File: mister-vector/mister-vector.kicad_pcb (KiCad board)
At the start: 4 copper layers, 68.6 x 106.6 mm, 120 parts, among them IC5 TL084, IC7 TL084, J2 AUDIO_JACK_3.5MM_KIT, U1 VASD1-SIP, U2 SN74LVC821ADGVR, U3 SN74LVC821ADGVR, U4 SN74LVC821ADGVR

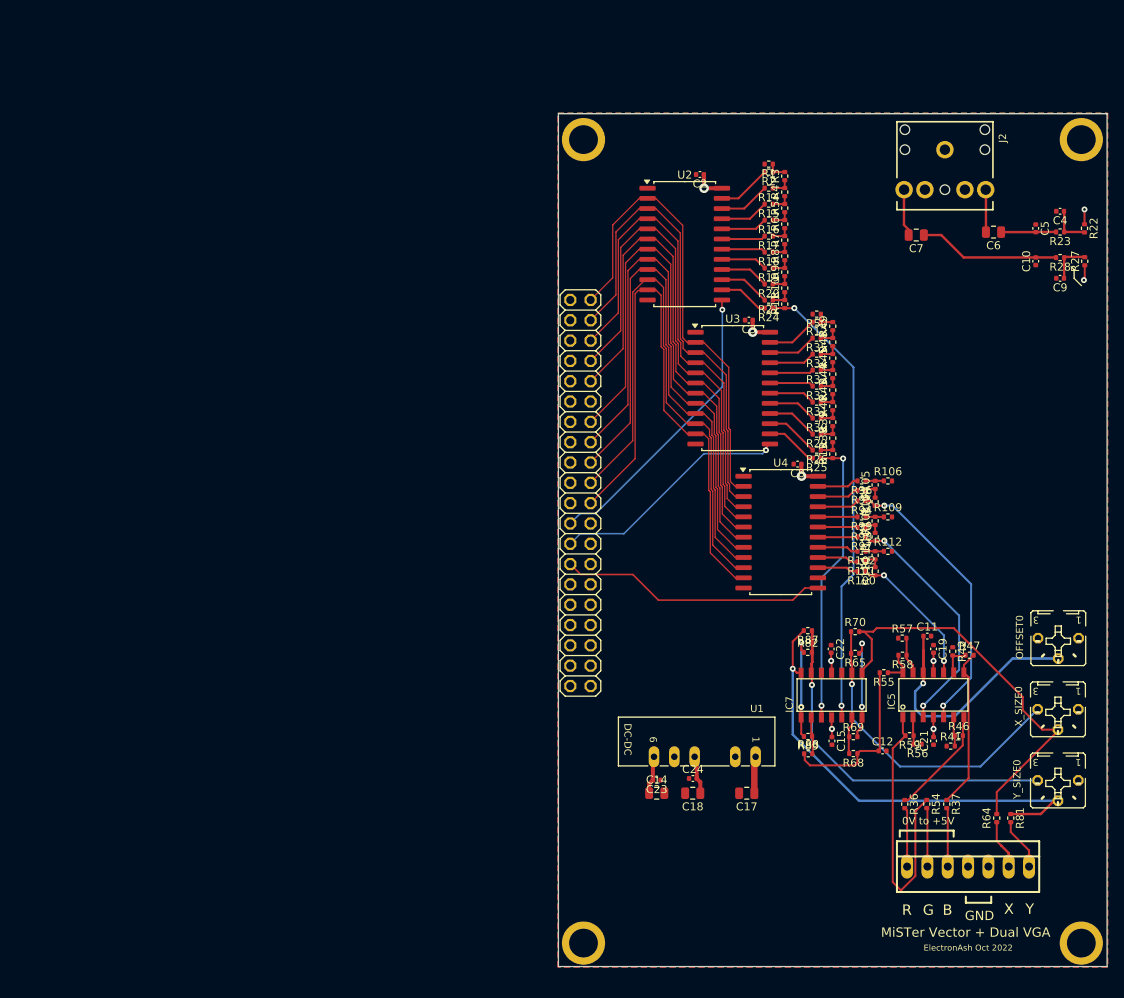
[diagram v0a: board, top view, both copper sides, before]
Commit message: update pcb screenshot
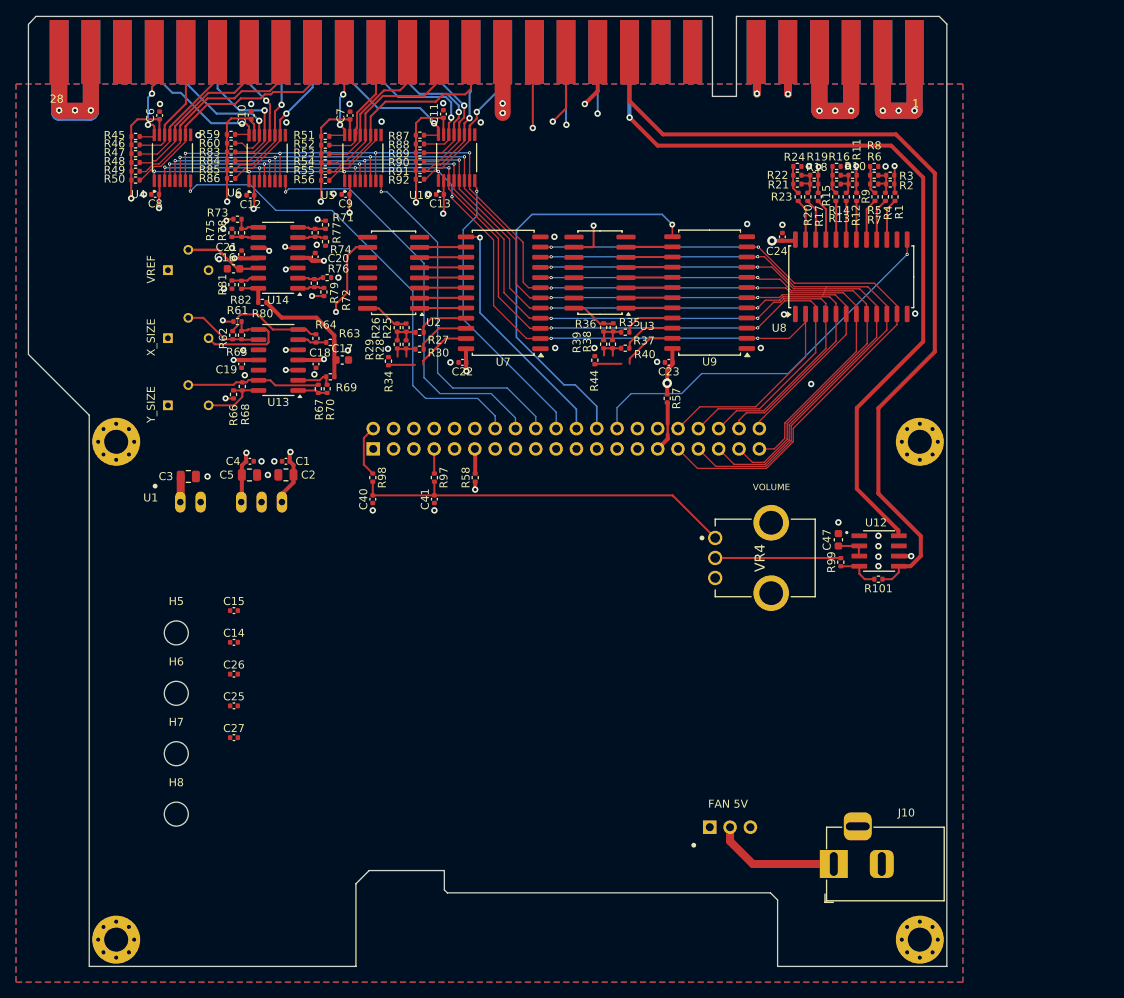
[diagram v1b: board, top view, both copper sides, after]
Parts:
- removed GPIO1: PINHD-2X20, 2X20
- removed IC5, IC7: TL084, SOIC-14
- removed J2: AUDIO_JACK_3.5MM_KIT, AUDIO-JACK-KIT
- removed OFFSET0, X_SIZE0, Y_SIZE0: 20K, B25P
- removed R100, R102, R106, R109, R112, R31, R32, R33, R94, R95, R96: 2k, Resistor_SMD:R_0402_1005Metric
- removed R104, R105, R107, R108, R110, R111, R43: 1k, Resistor_SMD:R_0402_1005Metric
- removed R41, R42: 10K, Resistor_SMD:R_0402_1005Metric
- removed U$1, U$2, U$3, U$4: PLATED_HOLE3.6MM, PLATED_HOLE_3.6MM
- removed VEC_OUT1: 22-23-2071, 22-23-2071
- added C1: 100nF, Capacitor_SMD:C_0402_1005Metric, F.Cu at (80.1, 95.1)
- added C13: 100nF, Capacitor_SMD:C_0402_1005Metric, F.Cu at (99.4, 61.8)
- added C16: 1uF, Capacitor_SMD:C_0603_1608Metric, F.Cu at (73.6, 71.1)
- added C20: 100nF, Capacitor_SMD:C_0402_1005Metric, F.Cu at (83.8, 69.6)
- added C25: 0.1pF, Capacitor_SMD:C_0402_1005Metric, F.Cu at (73.7, 125.7)
- added C26: 0.1pF, Capacitor_SMD:C_0402_1005Metric, F.Cu at (73.7, 121.8)
- added C27: 0.1pF, Capacitor_SMD:C_0402_1005Metric, F.Cu at (73.7, 129.7)
- added C40: 20nF, Capacitor_SMD:C_0402_1005Metric, F.Cu at (91.0, 99.9)
- added C41: 20nF, Capacitor_SMD:C_0402_1005Metric, F.Cu at (98.7, 99.9)
- added C47: 1uF, Capacitor_SMD:C_0603_1608Metric, F.Cu at (149.2, 105.0)
- added G***: LOGO, LOGO, F.Cu at (53.6, 56.7)
- added H1: MountingHole_Pad, MountingHole:MountingHole_3mm_Pad_Via, F.Cu at (159.4, 154.9)
- added H2: MountingHole_Pad, MountingHole:MountingHole_3mm_Pad_Via, F.Cu at (58.9, 92.7)
- added H3: MountingHole_Pad, MountingHole:MountingHole_3mm_Pad_Via, F.Cu at (159.4, 92.7)
- added H4: MountingHole_Pad, MountingHole:MountingHole_3mm_Pad_Via, F.Cu at (58.9, 154.9)
- added H5: FAN1, MountingHole:MountingHole_3mm, F.Cu at (66.4, 116.6)
- added H6: FAN2, MountingHole:MountingHole_3mm, F.Cu at (66.4, 124.2)
- added H7: FAN3, MountingHole:MountingHole_3mm, F.Cu at (66.4, 131.7)
- added H8: FAN4, MountingHole:MountingHole_3mm, F.Cu at (66.4, 139.2)
- added J10: DC-005-2.5A-2.0 C319099, Connector_BarrelJack:BarrelJack_Horizontal, F.Cu at (148.6, 145.5)
- added J100: FAN, Connector_PinHeader_2.54mm:PinHeader_1x03_P2.54mm_Vertical, F.Cu at (133.1, 140.9)
- added J7: PINHD-2X20, Connector_PinSocket_2.54mm:PinSocket_2x20_P2.54mm_Vertical, B.Cu at (91.1, 93.6)
- added J8: Jamma_con, Jamma:JAMMA-56, F.Cu at (158.9, 43.9)
- added R51: 100k, Resistor_SMD:R_0402_1005Metric, F.Cu at (85.1, 54.5)
- added R52: 100k, Resistor_SMD:R_0402_1005Metric, F.Cu at (85.1, 55.6)
- added R53: 100k, Resistor_SMD:R_0402_1005Metric, F.Cu at (85.1, 56.7)
- added R60: 100k, Resistor_SMD:R_0402_1005Metric, F.Cu at (73.3, 55.4)
- added R61: 75R, Resistor_SMD:R_0402_1005Metric, F.Cu at (74.1, 77.7)
- added R62: 75R, Resistor_SMD:R_0402_1005Metric, F.Cu at (73.5, 79.4)
- added R63: 10K, Resistor_SMD:R_0402_1005Metric, F.Cu at (85.7, 80.3)
- added R66: 75R, Resistor_SMD:R_0402_1005Metric, F.Cu at (73.6, 86.8)
- added R67: 75R, Resistor_SMD:R_0402_1005Metric, F.Cu at (84.2, 86.1)
- added R71: 75R, Resistor_SMD:R_0402_1005Metric, F.Cu at (85.1, 65.6)
- added R72: 75R, Resistor_SMD:R_0402_1005Metric, F.Cu at (84.9, 74.0)
- added R73: 75R, Resistor_SMD:R_0402_1005Metric, F.Cu at (74.1, 64.9)
- added R74: 10K, Resistor_SMD:R_0402_1005Metric, F.Cu at (85.1, 67.7)
- added R75: 10K, Resistor_SMD:R_0402_1005Metric, F.Cu at (73.4, 66.6)
- added R76: 10K, Resistor_SMD:R_0402_1005Metric, F.Cu at (85.3, 72.2)
- added R77: 4K7, Resistor_SMD:R_0402_1005Metric, F.Cu at (83.8, 66.6)
- added R78: 4K7, Resistor_SMD:R_0402_1005Metric, F.Cu at (74.6, 66.6)
- added R79: 4K7, Resistor_SMD:R_0402_1005Metric, F.Cu at (83.7, 72.9)
- added R80: 75R, Resistor_SMD:R_0402_1005Metric, F.Cu at (77.2, 75.3)
- added R83: 100k, Resistor_SMD:R_0402_1005Metric, F.Cu at (73.3, 56.5)
- added R84: 100k, Resistor_SMD:R_0402_1005Metric, F.Cu at (73.3, 57.6)
- added R85: 100k, Resistor_SMD:R_0402_1005Metric, F.Cu at (73.3, 58.7)
- added R86: 100k, Resistor_SMD:R_0402_1005Metric, F.Cu at (73.3, 59.8)
- added R90: 100k, Resistor_SMD:R_0402_1005Metric, F.Cu at (96.9, 57.7)
- added R91: 100k, Resistor_SMD:R_0402_1005Metric, F.Cu at (96.9, 58.8)
- added R92: 100k, Resistor_SMD:R_0402_1005Metric, F.Cu at (96.9, 59.9)
- added U10: TXB0106PWR, TXB0106PWR:SOP65P640X120-16N, F.Cu at (101.5, 57.2)
- added U12: LM4871MX_NOPB, LM4871MX_NOPB:SOIC127P599X175-8N, F.Cu at (154.3, 106.4)
- added U13: TL084HIDR, Package_SO:SOIC-14_3.9x8.7mm_P1.27mm, F.Cu at (79.2, 82.5)
- added U14: TL084HIDR, Package_SO:SOIC-14_3.9x8.7mm_P1.27mm, F.Cu at (79.2, 69.7)
- added U5: TXB0106PWR, TXB0106PWR:SOP65P640X120-16N, F.Cu at (89.8, 57.2)
- added U6: TXB0106PWR, TXB0106PWR:SOP65P640X120-16N, F.Cu at (77.8, 57.3)
- added U7: SN74LVC821ADGVR, Package_SO:SOIC-24W_7.5x15.4mm_P1.27mm, F.Cu at (107.3, 74.1)
- added U8: SN74LVC821ADGVR, Package_SO:SOIC-24W_7.5x15.4mm_P1.27mm, F.Cu at (150.8, 72.1)
- added U9: SN74LVC821ADGVR, Package_SO:SOIC-24W_7.5x15.4mm_P1.27mm, F.Cu at (133.1, 74.1)
- added VR1: VREF, 3362P_1_203LF:TRIM_3362P-1-203LF, F.Cu at (67.9, 71.3)
- added VR2: X_SIZE, 3362P_1_203LF:TRIM_3362P-1-203LF, F.Cu at (67.9, 79.8)
- added VR3: Y_SIZE, 3362P_1_203LF:TRIM_3362P-1-203LF, F.Cu at (67.9, 88.2)
- added VR4: 50k, PTV09A-4020U-A503:PTV09A4020FB103, F.Cu at (139.4, 107.2)
- C10, C4, C9: value 10nF -> 100nF
- C11, C12: value 1.0uF -> 100nF
- C14: value 4.7uF -> 0.1pF; footprint Capacitor_SMD:C_0805_2012Metric -> Capacitor_SMD:C_0402_1005Metric
- C15: value 100nF -> 0.1pF
- C17: value 4.7uF -> 1uF; footprint Capacitor_SMD:C_0805_2012Metric -> Capacitor_SMD:C_0603_1608Metric
- C18: value 4.7uF -> 100nF; footprint Capacitor_SMD:C_0805_2012Metric -> Capacitor_SMD:C_0402_1005Metric
- C2, C3: value 100nF -> 4.7uF; footprint Capacitor_SMD:C_0402_1005Metric -> Capacitor_SMD:C_0805_2012Metric
- C5: value 10nF -> 4.7uF; footprint Capacitor_SMD:C_0402_1005Metric -> Capacitor_SMD:C_0805_2012Metric
- C6, C7: value 4.7uF BP -> 100nF; footprint Capacitor_SMD:C_0805_2012Metric -> Capacitor_SMD:C_0402_1005Metric
- R1, R12, R14, R15, R16, R17, R18, R19, R2, R20, R21, R24, R25, R26, R29, R30, R34, R35: value 2k -> 100k 0.1%
- R10, R11, R13, R3, R38, R39, R4, R40, R44, R5, R6, R7, R8, R9: value 1k -> 100k 0.1%
- R101, R99: value 2k -> 20k
- R22, R23, R27, R28: value 510R -> 100k 0.1%
- R36, R37: value 75R -> 100k 0.1%
- R45, R48, R49: value 1k -> 100k
- R46, R47, R59: value 4K7 -> 100k
- R50: value 2k -> 100k
- R54, R55: value 75R -> 100k
- R56, R87, R88, R89: value 10K -> 100k
- R57: value 10K -> 0
- R58: value 4K7 -> 0
- R64, R65, R81: value 75R -> 10K
- R82: value 75R -> 4K7
- R97, R98: value 2k -> 475R
- U1: value VASD1-SIP -> RD-0512D
- U2, U3: value SN74LVC821ADGVR -> 4816P-R2R-503LF; footprint Package_SO:SOIC-24W_7.5x15.4mm_P1.27mm -> Package_SO:SOIC-16W_5.3x10.2mm_P1.27mm
- U4: value SN74LVC821ADGVR -> TXB0106PWR; footprint Package_SO:SOIC-24W_7.5x15.4mm_P1.27mm -> TXB0106PWR:SOP65P640X120-16N
- moved R46 126.7 mm to (61.4, 55.6), turned to 180 degrees
- moved R47 121.6 mm to (61.4, 56.7), turned to 180 degrees
- moved R81 118.0 mm to (73.4, 73.1), turned to 90 degrees
- moved R59 113.3 mm to (73.3, 54.3)
- moved R54 109.9 mm to (85.1, 57.8), turned to 180 degrees
- moved C4 106.0 mm to (75.6, 95.1)
- moved C21 105.7 mm to (74.6, 69.3), turned to -90 degrees
- moved C6 105.3 mm to (64.4, 51.9), turned to 90 degrees
- moved C12 105.2 mm to (75.7, 61.9), turned to 180 degrees
- moved R64 104.1 mm to (83.9, 79.8), turned to 90 degrees
- moved C5 103.0 mm to (75.6, 96.9), turned to 0 degrees
- moved R56 102.2 mm to (85.1, 60.0)
- moved C10 99.8 mm to (75.8, 51.9)
- moved R55 93.8 mm to (85.1, 58.9)
- moved C19 93.5 mm to (74.6, 83.0), turned to 90 degrees
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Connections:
- C10 pad 1: GND -> +5V
- C10 pad 2: Net-(C10-Pad2) -> GND
- C11 pad 1: Net-(IC5D-+IN) -> +5V
- C12 pad 1: /+VREF -> +3.3V
- C14 pad 1: +12V -> GND
- C14 pad 2: GND -> /Vector Amplifiers/DAC_B
- C15 pad 1: +12V -> GND
- C15 pad 2: GND -> /Vector Amplifiers/DAC_G
- C17 pad 1: +5V -> /Vector Amplifiers/+VREF
- C18 pad 1: -12V -> GND
- C18 pad 2: GND -> +12V
- C2 pad 1: +3.3V -> +12V
- C21 pad 2: +12V -> -12V
- C22 pad 1: GND -> +3.3V
- C22 pad 2: -12V -> GND
- C23 pad 1: GND -> +3.3V
- C23 pad 2: +12V -> GND
- C24 pad 1: GND -> +3.3V
- C24 pad 2: -12V -> GND
- C3 pad 1: +3.3V -> +5V
- C4 pad 1: Net-(C4-Pad1) -> GND
- C4 pad 2: GND -> -12V
- C5 pad 1: GND -> -12V
- C5 pad 2: Net-(C5-Pad2) -> GND
- C6 pad 1: Net-(C5-Pad2) -> +5V
- C6 pad 2: Net-(C6-Pad2) -> GND
- C7 pad 1: Net-(C10-Pad2) -> +5V
- C7 pad 2: Net-(C7-Pad2) -> GND
- C9 pad 1: Net-(C9-Pad1) -> +3.3V
- R1 pad 1: Net-(R1-Pad1) -> /Vector Amplifiers/DAC_B
- R1 pad 2: GND -> /Vector DACs/R2R_DAC_B/D2
- R10 pad 1: Net-(R10-Pad1) -> /Vector Amplifiers/DAC_G
- R101 pad 1: Net-(R101-Pad1) -> /JAMMA_SPEAKER+
- R101 pad 2: /R2R_DAC_B/D1 -> Net-(U12--IN)
- R11 pad 1: /DAC_X -> /Vector Amplifiers/DAC_G
- R11 pad 2: Net-(R10-Pad1) -> Net-(R10-Pad2)
- R12 pad 1: Net-(R12-Pad1) -> Net-(R10-Pad2)
- R12 pad 2: /R2R_DAC_Y/D0 -> /Vector DACs/R2R_DAC_G/D1
- R13 pad 1: /DAC_Y -> Net-(R10-Pad2)
- R14 pad 1: Net-(R14-Pad1) -> Net-(R10-Pad2)
- R14 pad 2: /R2R_DAC_X/D1 -> Net-(R13-Pad2)
- R15 pad 1: Net-(R15-Pad1) -> Net-(R13-Pad2)
- R15 pad 2: /R2R_DAC_X/D2 -> /Vector DACs/R2R_DAC_G/D0
- R16 pad 1: Net-(R16-Pad1) -> Net-(R13-Pad2)
- R16 pad 2: /R2R_DAC_X/D3 -> GND
- R17 pad 1: Net-(R17-Pad1) -> /Vector Amplifiers/DAC_R
- R17 pad 2: /R2R_DAC_X/D4 -> /Vector DACs/R2R_DAC_R/D2
- R18 pad 1: Net-(R18-Pad1) -> /Vector Amplifiers/DAC_R
- R18 pad 2: /R2R_DAC_X/D5 -> Net-(R18-Pad2)
- R19 pad 1: Net-(R19-Pad1) -> /Vector Amplifiers/DAC_R
- R19 pad 2: /R2R_DAC_X/D6 -> Net-(R18-Pad2)
- R2 pad 1: Net-(R1-Pad1) -> /Vector Amplifiers/DAC_B
- R2 pad 2: /R2R_DAC_X/D0 -> Net-(R2-Pad2)
- R20 pad 1: Net-(R10-Pad2) -> Net-(R18-Pad2)
- R20 pad 2: /R2R_DAC_X/D7 -> /Vector DACs/R2R_DAC_R/D1
- R21 pad 1: Net-(R10-Pad1) -> Net-(R18-Pad2)
- R21 pad 2: /R2R_DAC_X/D8 -> Net-(R21-Pad2)
- R22 pad 1: /AUDIO_R -> Net-(R18-Pad2)
- R22 pad 2: Net-(C4-Pad1) -> Net-(R21-Pad2)
- R23 pad 1: Net-(C4-Pad1) -> Net-(R21-Pad2)
- R23 pad 2: Net-(C5-Pad2) -> /Vector DACs/R2R_DAC_R/D0
- R24 pad 1: /DAC_X -> Net-(R21-Pad2)
- R24 pad 2: /R2R_DAC_X/D9 -> GND
- R25 pad 1: /DAC_Y -> Net-(R25-Pad1)
- R25 pad 2: /R2R_DAC_Y/D9 -> Net-(R25-Pad2)
- R26 pad 1: Net-(R13-Pad2) -> Net-(R25-Pad1)
- R26 pad 2: /R2R_DAC_Y/D8 -> Net-(R25-Pad2)
- R27 pad 1: /AUDIO_L -> Net-(R25-Pad2)
- R27 pad 2: Net-(C9-Pad1) -> /Vector DACs/R2R_DAC_X/D1
- R28 pad 1: Net-(C9-Pad1) -> Net-(R25-Pad2)
- R28 pad 2: Net-(C10-Pad2) -> Net-(R28-Pad2)
- R29 pad 1: Net-(R29-Pad1) -> Net-(R25-Pad2)
- R29 pad 2: /R2R_DAC_Y/D7 -> Net-(R28-Pad2)
- R3 pad 1: Net-(R14-Pad1) -> /Vector Amplifiers/DAC_B
- R3 pad 2: Net-(R1-Pad1) -> Net-(R2-Pad2)
- R30 pad 1: Net-(R30-Pad1) -> Net-(R28-Pad2)
- R30 pad 2: /R2R_DAC_Y/D6 -> /Vector DACs/R2R_DAC_X/D0
- R34 pad 1: Net-(R34-Pad1) -> Net-(R28-Pad2)
- R34 pad 2: /R2R_DAC_Y/D2 -> GND
- R35 pad 2: /R2R_DAC_Y/D1 -> Net-(R35-Pad2)
- R36 pad 1: Net-(IC5B-OUT) -> Net-(R35-Pad1)
- R36 pad 2: /R -> Net-(R35-Pad2)
- R37 pad 1: Net-(IC5C-OUT) -> Net-(R35-Pad2)
- R37 pad 2: /B -> /Vector DACs/R2R_DAC_Y/D1
- R38 pad 1: Net-(R13-Pad2) -> Net-(R35-Pad2)
- R38 pad 2: Net-(R29-Pad1) -> Net-(R38-Pad2)
- R39 pad 1: Net-(R29-Pad1) -> Net-(R35-Pad2)
- R39 pad 2: Net-(R30-Pad1) -> Net-(R38-Pad2)
- R4 pad 1: Net-(R15-Pad1) -> Net-(R2-Pad2)
- R4 pad 2: Net-(R14-Pad1) -> /Vector DACs/R2R_DAC_B/D1
- R40 pad 1: Net-(R30-Pad1) -> Net-(R38-Pad2)
- R40 pad 2: Net-(R31-Pad1) -> /Vector DACs/R2R_DAC_Y/D0
- R44 pad 1: Net-(R32-Pad1) -> Net-(R38-Pad2)
- R44 pad 2: Net-(R33-Pad1) -> GND
- R45 pad 1: Net-(R33-Pad1) -> /JAMMA_P1_BUTTON4
- R45 pad 2: Net-(R34-Pad1) -> +5V
- R46 pad 1: Net-(IC5B--IN) -> /JAMMA_P1_BUTTON3
- R46 pad 2: Net-(IC5B-OUT) -> +5V
- R47 pad 1: Net-(IC5C--IN) -> /JAMMA_P1_BUTTON2
- R47 pad 2: Net-(IC5C-OUT) -> +5V
- R48 pad 1: Net-(R34-Pad1) -> /JAMMA_P1_BUTTON1
- R48 pad 2: Net-(R35-Pad1) -> +5V
- R49 pad 1: Net-(R35-Pad1) -> /JAMMA_P1_R
- R49 pad 2: Net-(R12-Pad1) -> +5V
- R5 pad 1: Net-(R16-Pad1) -> Net-(R2-Pad2)
- R5 pad 2: Net-(R15-Pad1) -> Net-(R5-Pad2)
- R50 pad 1: Net-(R12-Pad1) -> /JAMMA_P1_L
- R50 pad 2: GND -> +5V
- R54 pad 1: Net-(IC5A-OUT) -> /JAMMA_P1_COIN
- R54 pad 2: /G -> +5V
- R55 pad 1: Net-(IC5D-OUT) -> /JAMMA_TEST
- R55 pad 2: /+VREF -> +5V
- R56 pad 1: GND -> /Input P1/I11
- R56 pad 2: Net-(IC5A--IN) -> +5V
- R57 pad 1: GND -> +3.3V
- R57 pad 2: Net-(IC5D--IN) -> Net-(J7-Pad29)
- R58 pad 1: Net-(IC5D--IN) -> +5V
- R58 pad 2: Net-(IC5D-OUT) -> Net-(J7-Pad11)
- R59 pad 1: Net-(IC5A--IN) -> /JAMMA_P2_BUTTON4
- R59 pad 2: Net-(IC5A-OUT) -> +5V
- R6 pad 1: Net-(R17-Pad1) -> Net-(R2-Pad2)
- R6 pad 2: Net-(R16-Pad1) -> Net-(R5-Pad2)
- R64 pad 1: Net-(IC7C-OUT) -> Net-(U13B--IN)
- R64 pad 2: /VEC_X -> Net-(U13B-OUT)
- R65 pad 1: Net-(IC7B-OUT) -> Net-(U13C--IN)
- R65 pad 2: Net-(IC7C--IN) -> Net-(U13C-OUT)
- R68 pad 1: /+VREF -> Net-(U13D--IN)
- R68 pad 2: Net-(IC7B--IN) -> Net-(U13D-OUT)
- R69 pad 1: Net-(IC7B--IN) -> /Vector Amplifiers/+VREF
- R69 pad 2: Net-(IC7B-OUT) -> Net-(U13A--IN)
- R7 pad 1: Net-(R18-Pad1) -> Net-(R5-Pad2)
- R7 pad 2: Net-(R17-Pad1) -> /Vector DACs/R2R_DAC_B/D0
- R70 pad 1: Net-(IC7C--IN) -> Net-(U13A--IN)
- R70 pad 2: Net-(IC7C-OUT) -> Net-(U13A-OUT)
- R8 pad 1: Net-(R19-Pad1) -> Net-(R5-Pad2)
- R8 pad 2: Net-(R18-Pad1) -> GND
- R81 pad 1: Net-(IC7D-OUT) -> GND
- R81 pad 2: /VEC_Y -> Net-(U14D--IN)
- R82 pad 1: Net-(IC7A-OUT) -> Net-(U14D--IN)
- R82 pad 2: Net-(IC7D--IN) -> Net-(U14D-OUT)
- R87 pad 1: Net-(IC7D--IN) -> /JAMMA_P2_D
- R87 pad 2: Net-(IC7D-OUT) -> +5V
- R88 pad 1: /+VREF -> /JAMMA_P2_U
- R88 pad 2: Net-(IC7A--IN) -> +5V
- R89 pad 1: Net-(IC7A--IN) -> /JAMMA_P2_START
- R89 pad 2: Net-(IC7A-OUT) -> +5V
- R9 pad 1: Net-(R10-Pad2) -> /Vector Amplifiers/DAC_G
- R9 pad 2: Net-(R19-Pad1) -> /Vector DACs/R2R_DAC_G/D2
- R97 pad 1: /DAC_G -> /AUDIO_R
- R97 pad 2: /R2R_DAC_G/D2 -> Net-(C40-Pad2)
- R98 pad 1: Net-(R107-Pad2) -> /AUDIO_L
- R98 pad 2: /R2R_DAC_G/D1 -> Net-(C40-Pad2)
- R99 pad 1: Net-(R108-Pad2) -> Net-(U12--IN)
- R99 pad 2: /R2R_DAC_G/D0 -> Net-(R99-Pad2)
- U2 pad 1: GND -> /Vector DACs/R2R_DAC_X/D2
- U2 pad 10: /D8 -> unconnected-(U2-Pad10)
- U2 pad 11: /D9 -> unconnected-(U2-Pad11)
- U2 pad 12: GND -> unconnected-(U2-Pad12)
- U2 pad 13: /CLK_X -> unconnected-(U2-Pad13)
- U2 pad 14: /R2R_DAC_X/D9 -> unconnected-(U2-Pad14)
- U2 pad 15: /R2R_DAC_X/D8 -> unconnected-(U2-Pad15)
- U2 pad 16: /R2R_DAC_X/D7 -> Net-(R25-Pad1)
- U2 pad 2: /D0 -> /Vector DACs/R2R_DAC_X/D3
- U2 pad 3: /D1 -> /Vector DACs/R2R_DAC_X/D4
- U2 pad 4: /D2 -> /Vector DACs/R2R_DAC_X/D5
- U2 pad 5: /D3 -> /Vector DACs/R2R_DAC_X/D6
- U2 pad 6: /D4 -> /Vector DACs/R2R_DAC_X/D7
- U2 pad 7: /D5 -> /Vector DACs/R2R_DAC_X/D8
- U2 pad 8: /D6 -> /Vector DACs/R2R_DAC_X/D9
- U2 pad 9: /D7 -> /Vector Amplifiers/DAC_X
- U3 pad 1: GND -> /Vector DACs/R2R_DAC_Y/D2
- U3 pad 10: /D8 -> unconnected-(U3-Pad10)
- U3 pad 11: /D9 -> unconnected-(U3-Pad11)
- U3 pad 12: GND -> unconnected-(U3-Pad12)
- U3 pad 13: /CLK_Y -> unconnected-(U3-Pad13)
- U3 pad 14: /R2R_DAC_Y/D9 -> unconnected-(U3-Pad14)
- U3 pad 15: /R2R_DAC_Y/D8 -> unconnected-(U3-Pad15)
- U3 pad 16: /R2R_DAC_Y/D7 -> Net-(R35-Pad1)
- U3 pad 2: /D0 -> /Vector DACs/R2R_DAC_Y/D3
- U3 pad 3: /D1 -> /Vector DACs/R2R_DAC_Y/D4
- U3 pad 4: /D2 -> /Vector DACs/R2R_DAC_Y/D5
- U3 pad 5: /D3 -> /Vector DACs/R2R_DAC_Y/D6
- U3 pad 6: /D4 -> /Vector DACs/R2R_DAC_Y/D7
- U3 pad 7: /D5 -> /Vector DACs/R2R_DAC_Y/D8
- U3 pad 8: /D6 -> /Vector DACs/R2R_DAC_Y/D9
- U3 pad 9: /D7 -> /Vector Amplifiers/DAC_Y
- U4 pad 1: GND -> /D0
- U4 pad 10: /D8 -> /JAMMA_P1_L
- U4 pad 11: /D9 -> /JAMMA_P1_R
- U4 pad 12: GND -> /JAMMA_P1_BUTTON1
- U4 pad 13: /CLK_RGB -> /JAMMA_P1_BUTTON2
- U4 pad 14: unconnected-(U4-10Q-Pad14) -> /JAMMA_P1_BUTTON3
- U4 pad 15: /R2R_DAC_B/D2 -> +5V
- U4 pad 16: /R2R_DAC_B/D1 -> /JAMMA_P1_BUTTON4
- U4 pad 2: /D0 -> +3.3V
- U4 pad 8: /D6 -> /CLK_P10
- U4 pad 9: /D7 -> GND
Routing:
- net +5V: track 52.4 -> 407.8 mm, vias 0 -> 9
- net /JAMMA_SPEAKER+: track 0.00 -> 106.8 mm
- net /JAMMA_SPEAKER-: track 0.00 -> 98.3 mm, vias 0 -> 1
- net /Vector Amplifiers/DAC_B: track 0.00 -> 96.5 mm, vias 0 -> 2
- net /JAMMA_PIN_11(Y): track 0.00 -> 89.4 mm, vias 0 -> 2
- net /AUDIO_R: track 86.2 -> 3.05 mm, vias 1 -> 0
- net /Vector Amplifiers/DAC_G: track 0.00 -> 81.6 mm, vias 0 -> 2
- net /AUDIO_L: track 87.2 -> 6.59 mm, vias 1 -> 0
- net /JAMMA_PIN_M(X): track 0.00 -> 78.8 mm, vias 0 -> 2
- net GND: track 0.00 -> 77.2 mm, vias 0 -> 56
- net /Vector Amplifiers/DAC_R: track 0.00 -> 75.7 mm, vias 0 -> 2
- net /D0: track 59.6 -> 128.8 mm, vias 0 -> 7
- net /D2: track 62.2 -> 130.0 mm, vias 0 -> 6
- net /D1: track 60.9 -> 128.0 mm, vias 0 -> 6
- net /D5: track 68.5 -> 133.0 mm, vias 0 -> 6
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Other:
- board size 68.6 x 106.6 mm -> 114.8 x 118.8 mm
- board text added: "FAN 5V"
- board text added: "MISTER VECTOR JAMMA V1.0 ©2025"
- board text added: "VOLUME"
- board text removed: "0V to +5V"
- board text removed: "B"
- board text removed: "ElectronAsh Oct 2022"
- board text removed: "G"
- board text removed: "GND"
- board text removed: "MiSTer Vector + Dual VGA"
- board text removed: "X"
- board text removed: "Y"
